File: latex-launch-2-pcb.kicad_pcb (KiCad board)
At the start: 4 copper layers, 82.6 x 66.3 mm, 14 parts, among them J1 Conn_RockBLOCK, J2 Switch_RockBLOCK, J3 Conn_FeatherWeight, J4 Conn_LightAPRS, J5 Conn_MicroSD, J6 Conn_GY-512_MPU6050

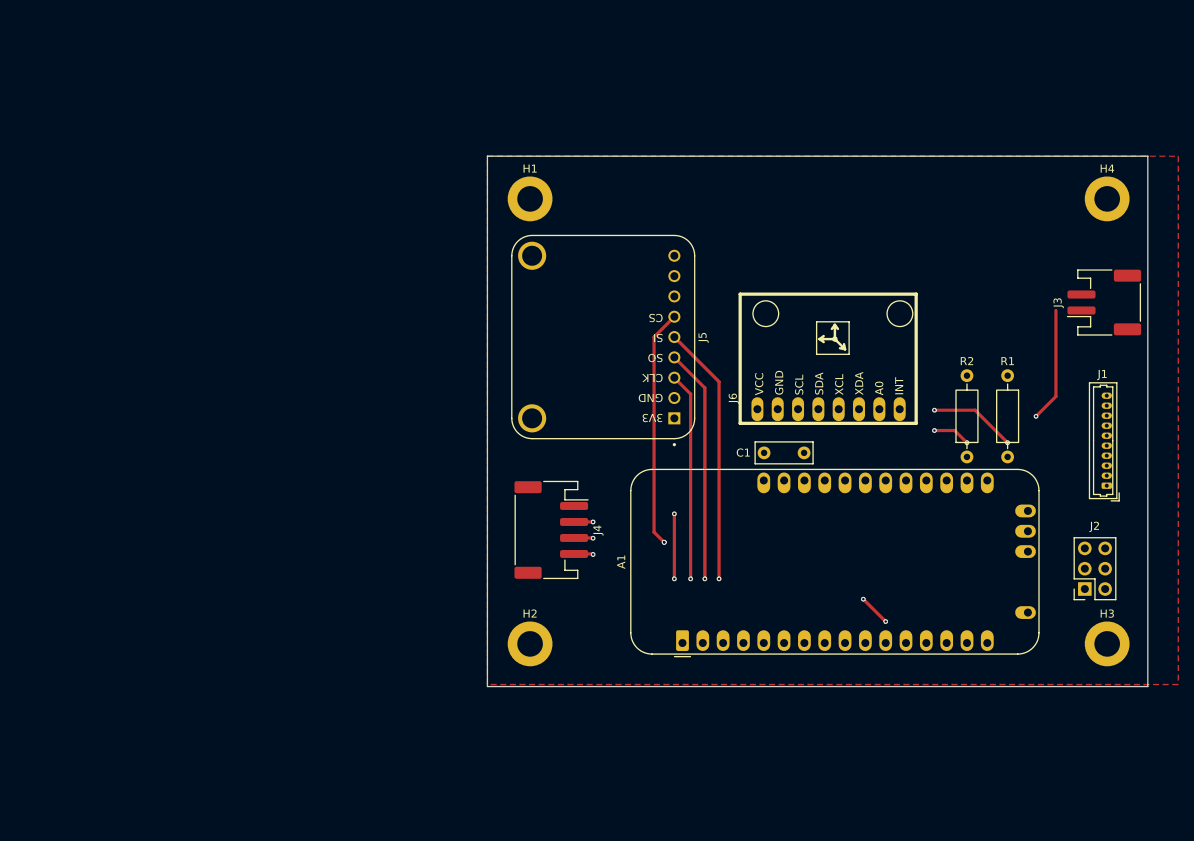
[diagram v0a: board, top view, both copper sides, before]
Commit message: better pcb
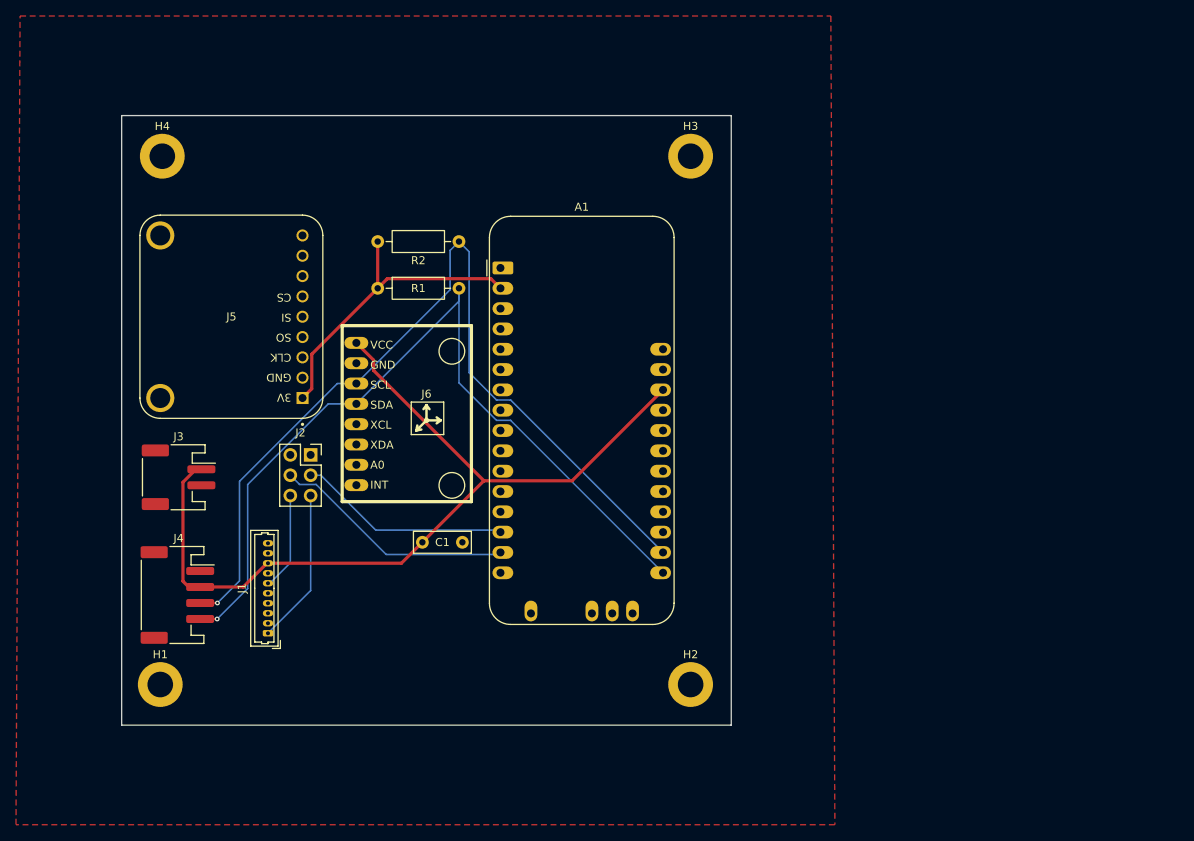
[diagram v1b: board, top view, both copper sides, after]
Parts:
- moved H4 118.2 mm to (68.6, 68.6)
- moved J3 117.8 mm to (70.6, 108.7), turned to -90 degrees
- moved J1 106.5 mm to (81.8, 128.2)
- moved J2 98.2 mm to (87.1, 105.9), turned to 0 degrees
- moved H3 80.2 mm to (134.6, 68.6)
- moved R1 79.5 mm to (95.5, 85.1), turned to 0 degrees
- moved H1 76.3 mm to (68.3, 134.6)
- moved R2 69.0 mm to (105.7, 79.2), turned to 180 degrees
- moved A1 52.1 mm to (110.9, 82.5), turned to 0 degrees
- moved J6 52.1 mm to (101.6, 101.6), turned to 0 degrees
- moved C1 49.0 mm to (101.1, 116.8), turned to 0 degrees
- moved J4 47.4 mm to (70.5, 123.4)
- moved J5 46.6 mm to (77.2, 88.6)
- moved H2 20.7 mm to (134.6, 134.6)
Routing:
- net +3V3: track 73.4 -> 39.8 mm, vias 2 -> 0
- net /I2C_SCL: track 82.8 -> 111.7 mm, vias 3 -> 1
- net /SPI_MISO: track 60.3 -> 34.1 mm, vias 1 -> 0
- net /SPI_MOSI: track 59.3 -> 34.3 mm, vias 3 -> 0
- net /I2C_SDA: track 90.7 -> 105.4 mm, vias 3 -> 1
- net +BATT: track 96.5 -> 109.7 mm, vias 2 -> 0
- net /SPI_SCK: track 53.7 -> 42.0 mm, vias 1 -> 0
- net /CS_SDCard: track 68.3 -> 57.3 mm, vias 2 -> 0
- net /Rx_RockBLOCK: track 8.97 -> 19.4 mm
- net /Tx: track 21.1 -> 30.5 mm
- net /Rx: track 21.1 -> 26.7 mm
- net /Tx_RockBLOCK: track 15.3 -> 12.3 mm
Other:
- board size 82.6 x 66.3 mm -> 76.2 x 76.2 mm

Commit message: PCB version 2
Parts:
- removed H1, H2, H3, H4: MountingHole, MountingHole:MountingHole_3.2mm_M3_DIN965_Pad
- added J7: Conn_MicroSD, Latex Launch 2 Footprints:Adafruit_MicroSD_Breakout, F.Cu at (228.6, 113.0)
- added J8: Conn_HTU21DF, Latex Launch 2 Footprints:Adafruit_HTU21DF_Breakout, F.Cu at (174.1, 117.5)
- added R3: R_shunt, Connector_PinHeader_2.54mm:PinHeader_1x02_P2.54mm_Vertical, F.Cu at (201.9, 67.3)
- added R4: R_shunt, Connector_PinHeader_2.54mm:PinHeader_1x02_P2.54mm_Vertical, F.Cu at (207.3, 67.3)
- added U1: ~, Latex Launch 2 Footprints:Adafruit_RFM96W_LoRa_Breakout, F.Cu at (200.6, 110.7)
- A1: value Adafruit_Feather_M0_RFM9x_LoRa_Radio -> Adafruit_Feather_M0_Express; footprint Module:Adafruit_Feather_M0_RFM -> Module:Adafruit_Feather_M0_RFM_WithMountingHoles
- C1: value C0.1u -> C; footprint Capacitor_THT:C_Rect_L7.0mm_W2.5mm_P5.00mm -> Capacitor_THT:C_Rect_L4.6mm_W2.0mm_P2.50mm_MKS02_FKP02
- J1: value Conn_RockBLOCK -> Conn_GPS; footprint Connector_Molex:Molex_PicoBlade_53047-1010_1x10_P1.25mm_Vertical -> Latex Launch 2 Footprints:Adafruit_GPS_Breakout
- J2: value Switch_RockBLOCK -> Conn_LightAPRS-W_2.0; footprint Connector_PinSocket_2.54mm:PinSocket_2x03_P2.54mm_Vertical -> Connector_JST:JST_PH_S4B-PH-SM4-TB_1x04-1MP_P2.00mm_Horizontal
- J4: value Conn_LightAPRS -> Conn_RockBLOCK; footprint Connector_JST:JST_PH_S4B-PH-SM4-TB_1x04-1MP_P2.00mm_Horizontal -> Connector_Molex:Molex_PicoBlade_53047-1010_1x10_P1.25mm_Vertical
- J5: value Conn_MicroSD -> Conn_GY512_MPU6050; footprint Module:Adafruit_MicroSD_Breakout -> Latex Launch 2 Footprints:GY-521 MPU6050
- J6: value Conn_GY-512_MPU6050 -> Conn_BMP280; footprint Module:GY-521 MPU6050 -> Latex Launch 2 Footprints:Adafruit_BMP280_Breakout
- R1, R2: value R10k -> 10k
- moved J4 174.3 mm to (230.4, 54.0), turned to 90 degrees
- moved J1 150.7 mm to (224.8, 80.5), turned to 180 degrees
- moved J5 126.1 mm to (203.2, 82.5), turned to 0 degrees
- moved J3 104.7 mm to (172.2, 83.6)
- moved R1 96.1 mm to (190.5, 70.9), turned to 180 degrees
- moved J2 92.3 mm to (172.2, 70.1), turned to -90 degrees
- moved C1 88.2 mm to (168.7, 60.2)
- moved R2 86.1 mm to (190.5, 64.5)
- moved J6 75.0 mm to (176.5, 99.3), turned to 90 degrees
- moved A1 72.9 mm to (180.3, 60.6), turned to 90 degrees
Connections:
- A1 pad 14: /Rx -> Net-(A1-RX/D0)
- A1 pad 15: /Tx -> Net-(A1-TX/D1)
- A1 pad 19: /CS_SDCard -> /CS_SD
- A1 pad 20: unconnected-(A1-D6-Pad20) -> /EN_GPS
- A1 pad 21: unconnected-(A1-D9-Pad21) -> /EN_RockBLOCK
- A1 pad 22: unconnected-(A1-D10-Pad22) -> /CS_RFM96W
- A1 pad 23: unconnected-(A1-D11-Pad23) -> /CS_BMP280
- A1 pad 26: +BATT -> unconnected-(A1-USB-Pad26)
- A1 pad 28: unconnected-(A1-VBAT-Pad28) -> +BATT
- A1 pad 29: unconnected-(A1-ANT-Pad29) -> (no net)
- A1 pad 30: unconnected-(A1-DIO5-Pad30) -> (no net)
- A1 pad 31: unconnected-(A1-DIO3-Pad31) -> (no net)
- A1 pad 32: unconnected-(A1-DIO2-Pad32) -> (no net)
- J1 pad 1: /Rx_RockBLOCK -> unconnected-(J1-Pin_1-Pad1)
- J1 pad 2: unconnected-(J1-Pin_2-Pad2) -> /EN_GPS
- J1 pad 5: unconnected-(J1-Pin_5-Pad5) -> /Rx_iso
- J1 pad 6: /Tx_RockBLOCK -> /Tx_iso
- J1 pad 7: unconnected-(J1-Pin_7-Pad7) -> GND
- J1 pad 8: +BATT -> +3V3
- J2 pad 1: unconnected-(J2-Pin_1-Pad1) -> /I2C_SCL
- J2 pad 2: unconnected-(J2-Pin_2-Pad2) -> /I2C_SDA
- J2 pad 3: /Rx -> +BATT
- J2 pad 4: /Tx -> GND
- J3 pad 1: +BATT -> +3V3
- J4 pad 1: GND -> /Rx_iso
- J4 pad 2: +BATT -> unconnected-(J4-Pin_2-Pad2)
- J4 pad 3: /I2C_SCL -> unconnected-(J4-Pin_3-Pad3)
- J4 pad 4: /I2C_SDA -> unconnected-(J4-Pin_4-Pad4)
- J5 pad 3: /SPI_SCK -> /I2C_SCL
- J5 pad 4: /SPI_MISO -> /I2C_SDA
- J5 pad 5: /SPI_MOSI -> unconnected-(J5-Pin_5-Pad5)
- J5 pad 6: /CS_SDCard -> unconnected-(J5-Pin_6-Pad6)
- J6 pad 1: +BATT -> +3V3
- J6 pad 2: GND -> unconnected-(J6-Pin_2-Pad2)
- J6 pad 3: /I2C_SCL -> GND
- J6 pad 4: /I2C_SDA -> /SPI_SCK
- J6 pad 5: unconnected-(J6-Pin_5-Pad5) -> /SPI_MISO
- J6 pad 6: unconnected-(J6-Pin_6-Pad6) -> /SPI_MOSI
- J6 pad 7: unconnected-(J6-Pin_7-Pad7) -> /CS_BMP280
- R2 pad 1: /I2C_SCL -> +3V3
- R2 pad 2: +3V3 -> /I2C_SCL
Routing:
- net +3V3: track 39.8 -> 148.8 mm, vias 0 -> 1
- net /CS_SD: track 0.00 -> 78.9 mm
- net /CS_RFM96W: track 0.00 -> 64.7 mm
- net /CS_BMP280: track 0.00 -> 59.6 mm
- net /SPI_MOSI: track 34.3 -> 92.1 mm, vias 0 -> 2
- net /CS_SDCard: track 57.3 -> 0.00 mm
- net /SPI_MISO: track 34.1 -> 89.1 mm, vias 0 -> 2
- net /SPI_SCK: track 42.0 -> 94.0 mm
- net /EN_GPS: track 0.00 -> 42.9 mm
- net /Rx_iso: track 0.00 -> 38.6 mm
- net /Tx_iso: track 0.00 -> 37.1 mm
- net /Tx: track 30.5 -> 0.00 mm
- net /EN_RockBLOCK: track 0.00 -> 29.6 mm
- net /Rx: track 26.7 -> 0.00 mm
- net +BATT: track 109.7 -> 86.6 mm
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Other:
- board size 76.2 x 76.2 mm -> 76.2 x 88.9 mm
